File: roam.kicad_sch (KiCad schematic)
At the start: 301 parts, among them IC2 MCP73833T-FCI/MF, J1 SIM8060-6-0-14-00-A, J2 Battery, J3 Conn_01x03_Pin, J4 USB_B_Micro, J5 Conn_01x03_Pin, J7 MX23A18NF1, Q2 MMBT3904, Q3 MMBT3904, Q5 BC846A,215, Q6 BC846A,215, Q7 BC846A,215, U10 LTV-217, U11 MAX13487EESAT, U12 LM3671MF-3.3/NOPB, U13 LIS2DH12TR, U14 MAX17643ATC+, U15 FDMC86139P, U16 MCP2562-E/MF, U17 LTV-217, U18 MP3423GG, U2 MDBT50Q-1M, U20 TPS566242DRLR, U23 TXS0102DCU, U24 LP5907MFX-3.3, U27 EG915ULAAB-N05-SNNSA, U28 LC29H, U29 USBLC6-2SC6, U3 TXB0108DQSR, U31 B8389, U32 LP5907MFX-3.3, U4 STM32F105RBT6, U6 MCP2562-E/MF, U6 MX25R6435FZNIL0, U6 W25N512GVEIG, U7 LM66100DCKR, U8 GP.1575.25.2.A.02, U9 LM66100DCKR, Y1 25MHz

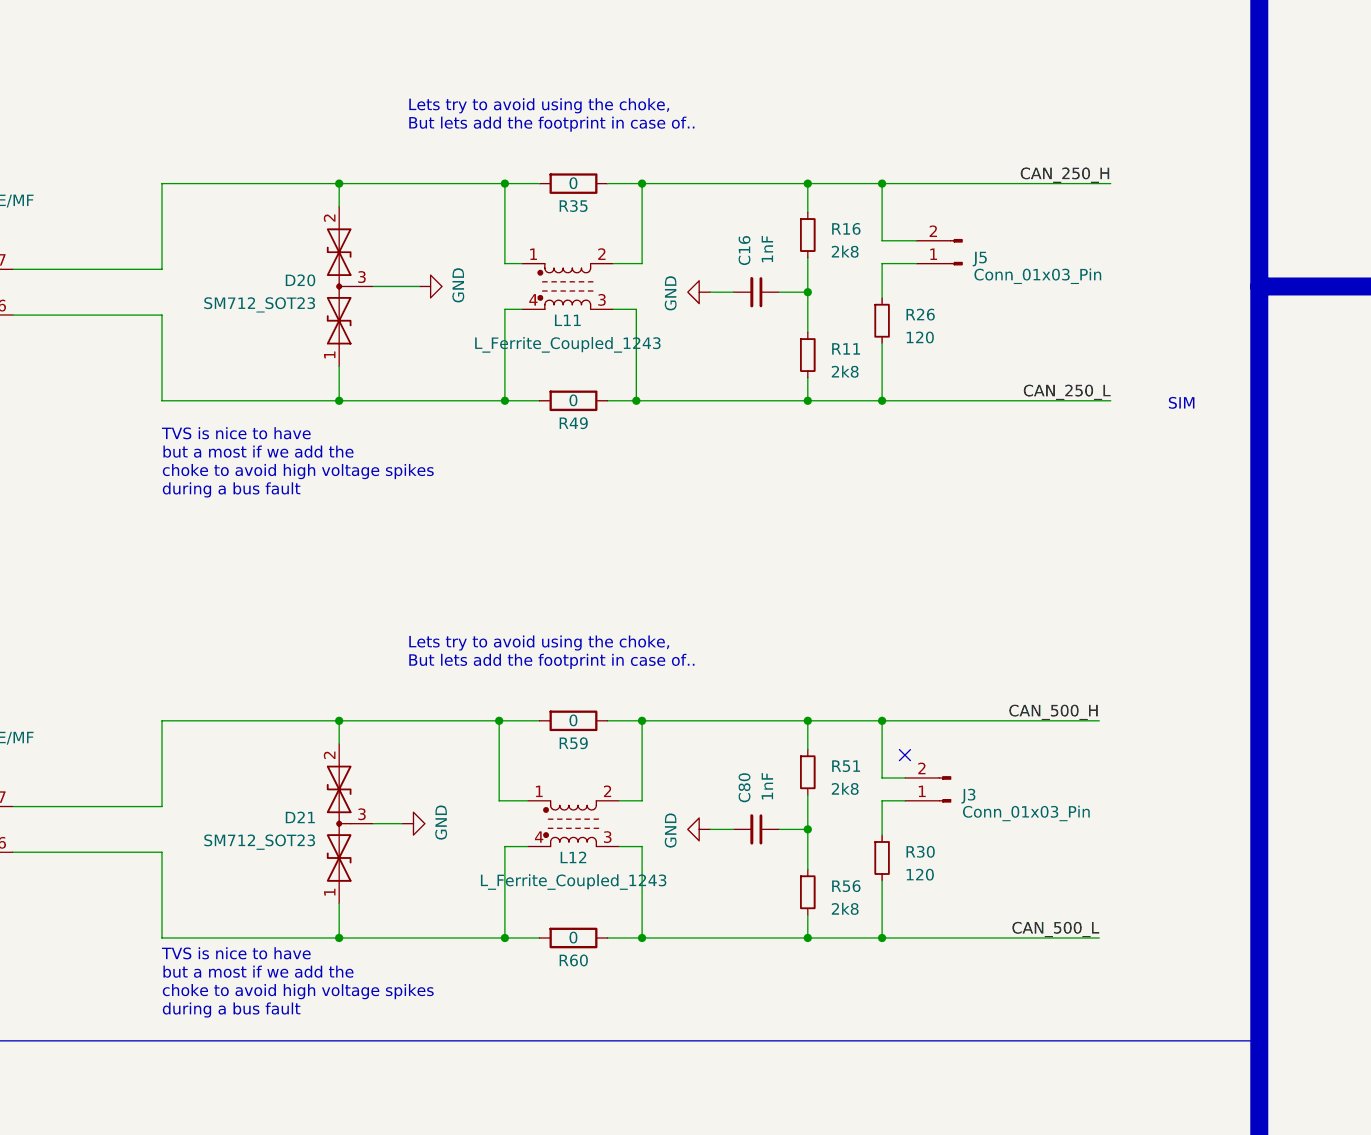
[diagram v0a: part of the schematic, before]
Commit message: updated 4/12
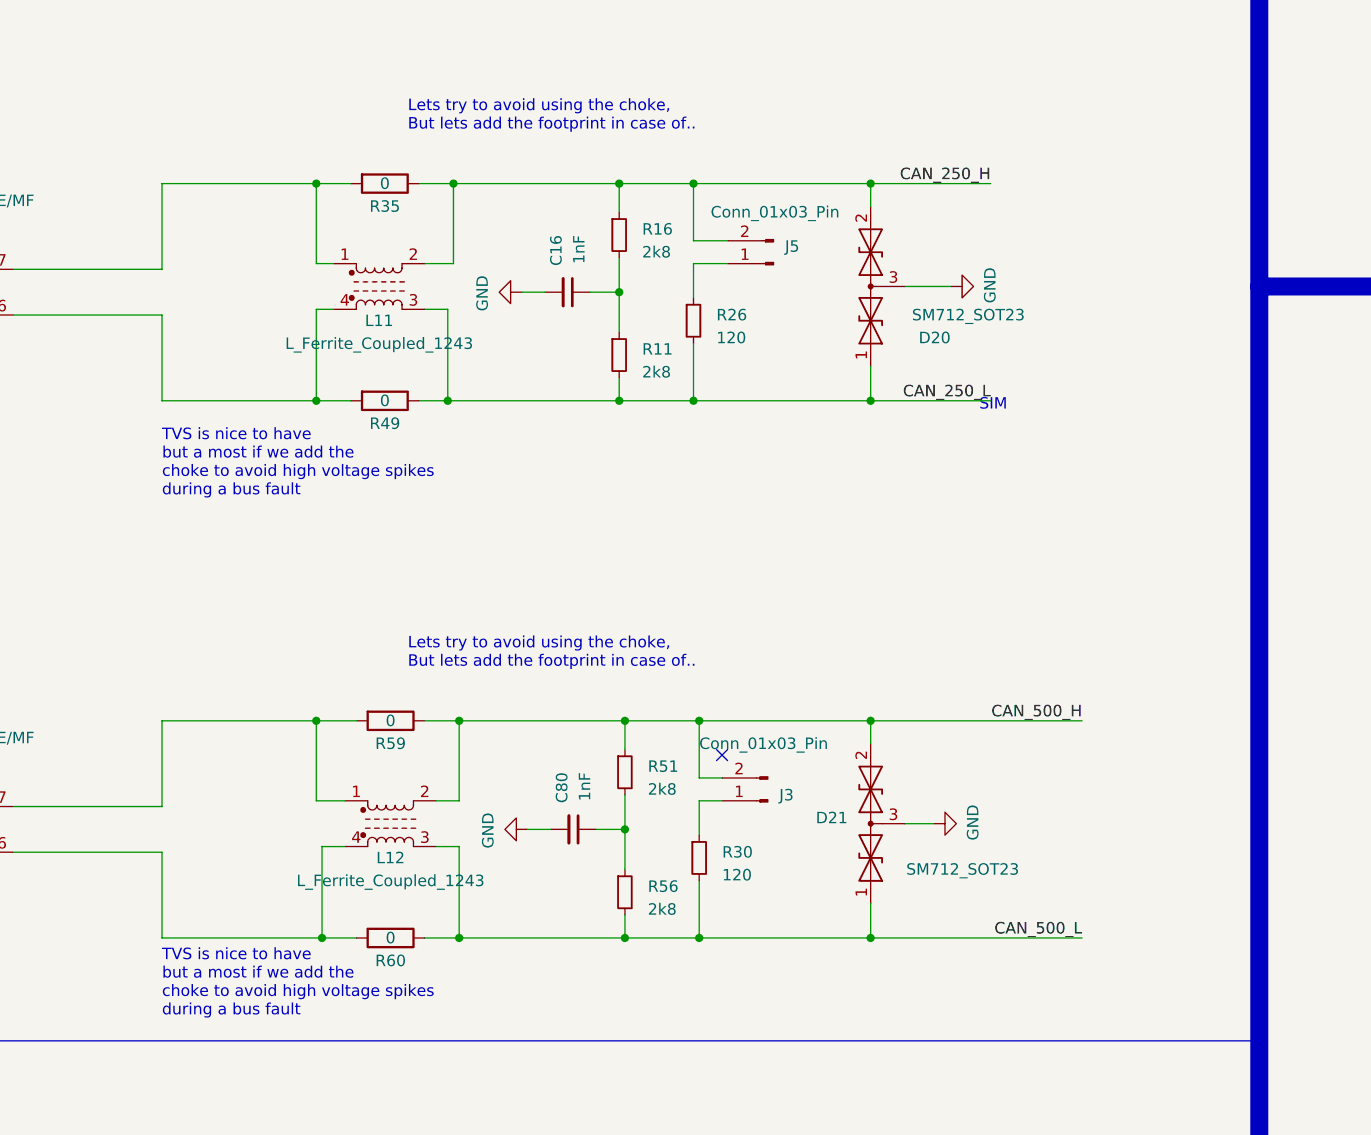
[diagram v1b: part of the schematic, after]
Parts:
- J3: footprint Connector_PinHeader_1.27mm:PinHeader_1x02_P1.27mm_Vertical_SMD_Pin1Right -> Connector_PinHeader_1.27mm:PinHeader_1x02_P1.27mm_Vertical_SMD_Pin1Left
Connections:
- net CAN_250_H: now also D20.2 (A2)
- net CAN_250_L: now also D20.1 (A1)
- net CAN_500_H: now also D21.2 (A2)
- net CAN_500_L: now also D21.1 (A1)
- net at L12.1, R59.2, U16.7 (CANH): no longer D21.2 (A2)
- net at L12.4, R60.2, U16.6 (CANL): no longer D21.1 (A1)
- net at L11.4, R49.2, U6.6 (CANL): no longer D20.1 (A1)
- net at L11.1, R35.2, U6.7 (CANH): no longer D20.2 (A2)
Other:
- moved on the sheet: C16, C80, J3, J5, L11, L12, R11, R16, R26, R30, R35, R49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
